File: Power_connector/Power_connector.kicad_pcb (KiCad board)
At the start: 2 copper layers, 107.2 x 80.8 mm, 65 parts, among them J1 XT60_F, J10 XT60_F, J11 XT60_F, J12 XT60_F, J13 XT60_F, J14 XT60_F, J2 XT60_Male, J3 XT60_F, J4 E_Stop, J5 XT60_F, J6 XT60_F, J7 XT60_F, J8 XT60_F, J9 XT60_F, Q1 IRFS7530, Q2 IRFS7530

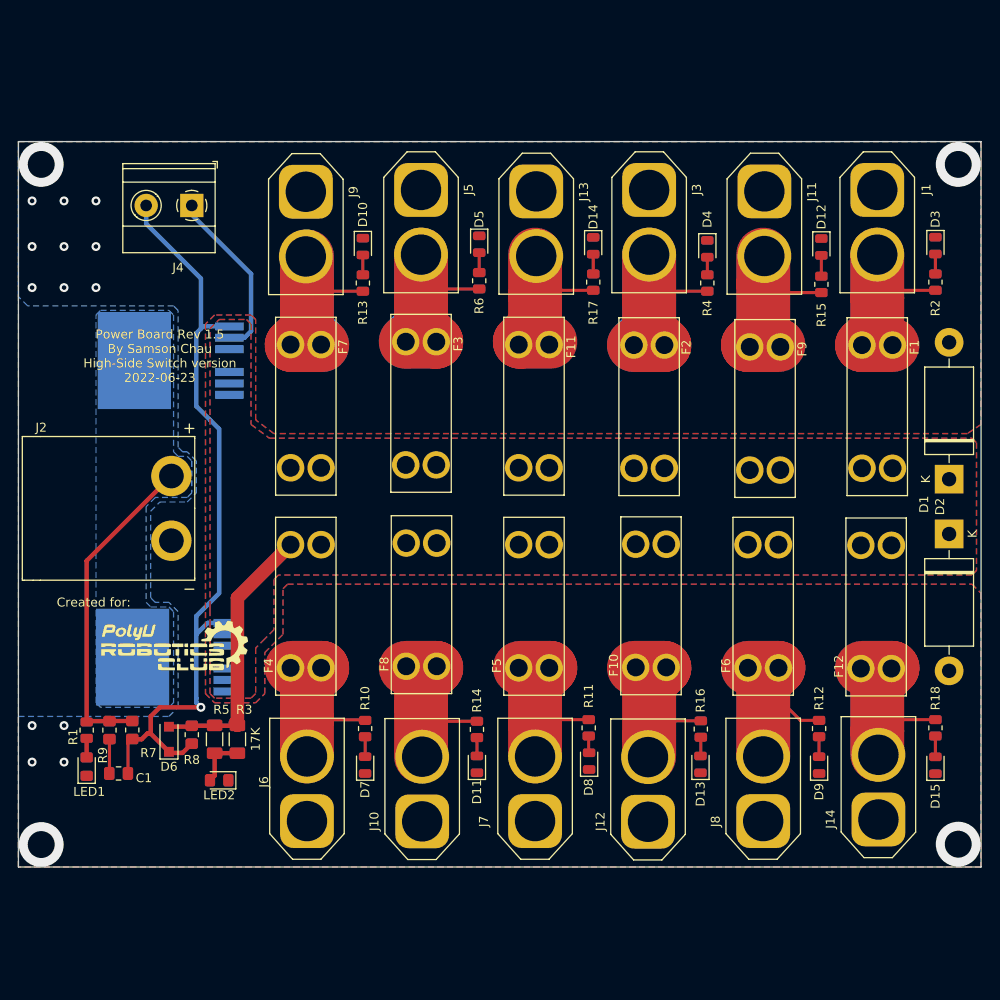
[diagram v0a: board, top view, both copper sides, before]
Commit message: new shield
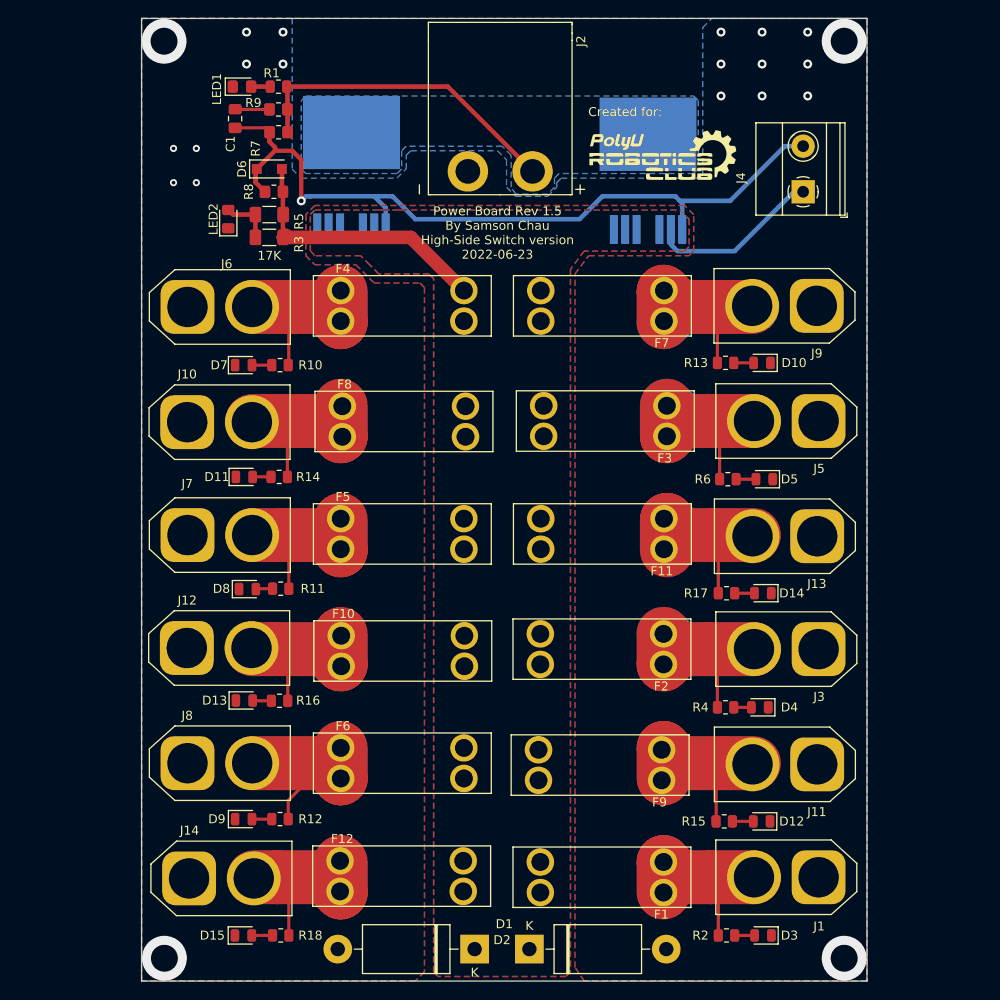
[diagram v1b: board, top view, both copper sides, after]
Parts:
- moved D15 79.4 mm to (101.2, 142.7), turned to 0 degrees
- moved D3 79.2 mm to (159.1, 142.7), turned to 180 degrees
- moved LED1 77.7 mm to (101.1, 48.2), turned to 0 degrees
- moved G*** 77.1 mm to (148.1, 56.1)
- moved J14 77.0 mm to (95.2, 136.4), turned to 0 degrees
- moved J1 76.8 mm to (165.3, 136.3), turned to 180 degrees
- moved R18 76.5 mm to (105.4, 142.7), turned to 180 degrees
- moved R2 76.4 mm to (155.0, 142.7), turned to 0 degrees
- moved R1 74.8 mm to (105.2, 48.2), turned to 180 degrees
- moved C1 74.1 mm to (100.3, 51.8), turned to -90 degrees
- moved R9 71.6 mm to (105.2, 50.8), turned to 180 degrees
- moved D2 70.2 mm to (127.0, 144.3), turned to 180 degrees
- moved D1 70.2 mm to (133.1, 144.3), turned to 0 degrees
- moved R7 68.5 mm to (105.2, 53.3), turned to 180 degrees
- moved J4 68.1 mm to (163.6, 59.9), turned to 90 degrees
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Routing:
- net GND: vias 13 -> 17
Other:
- board size 107.2 x 80.8 mm -> 80.8 x 107.2 mm
